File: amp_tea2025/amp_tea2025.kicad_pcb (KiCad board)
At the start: 2 copper layers, 18 parts, among them J1 in, J2 SPK, J3 SPK, U1 TEA2025

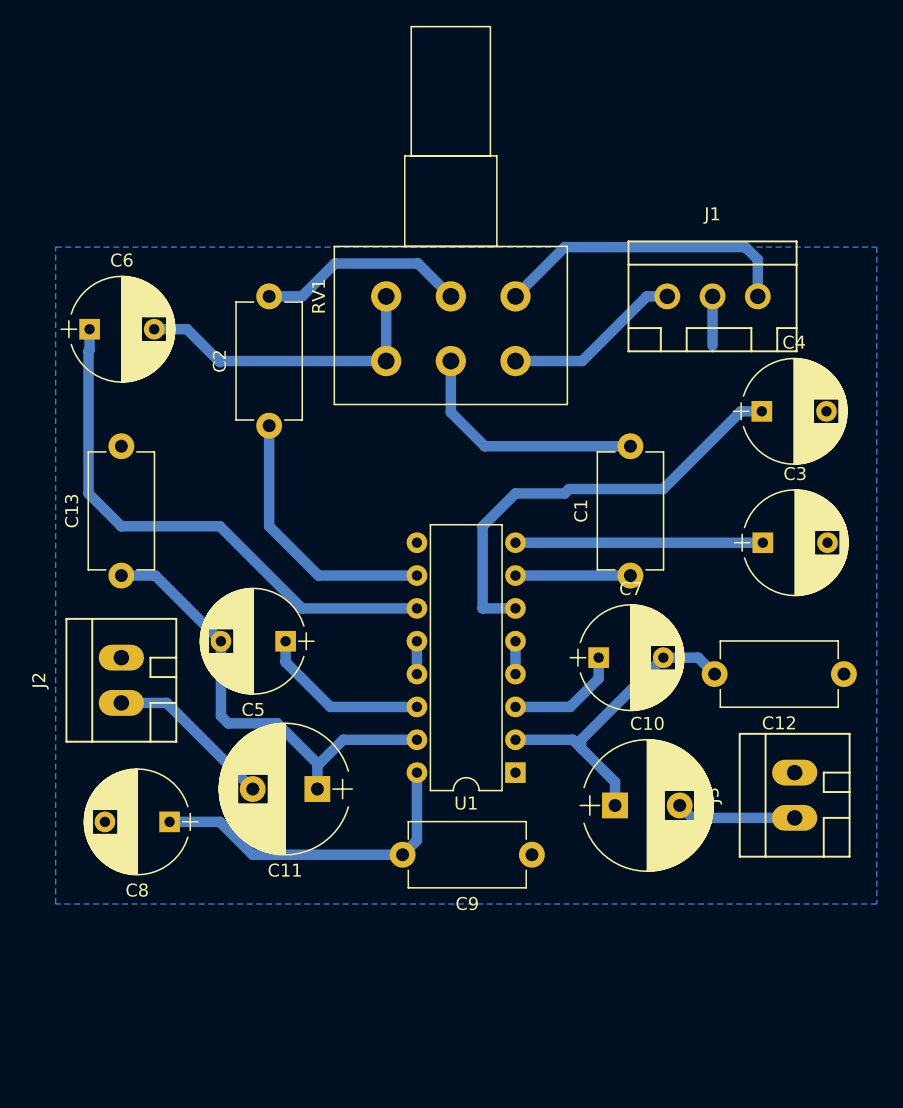
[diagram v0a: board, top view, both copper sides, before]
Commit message: pdf
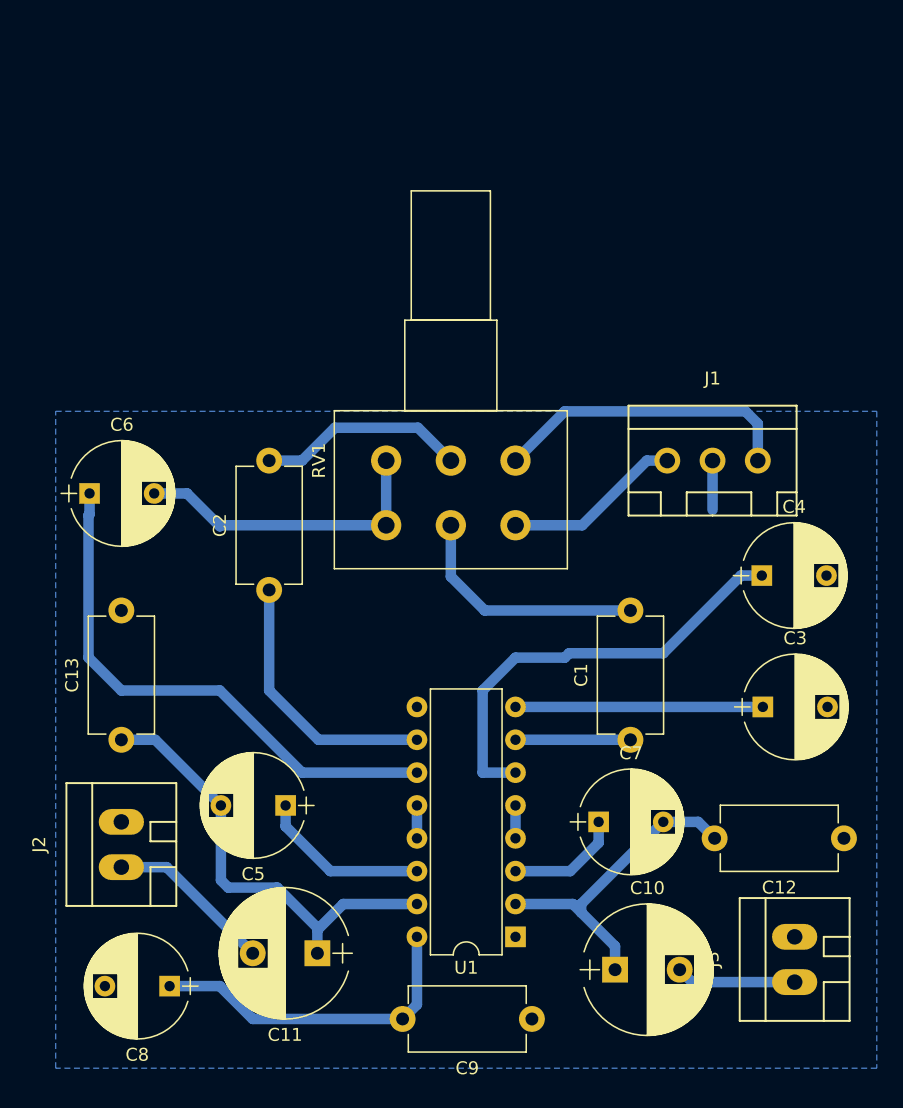
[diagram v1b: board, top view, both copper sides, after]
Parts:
- moved C11 12.7 mm to (45.6, 67.3)
- moved C12 12.7 mm to (86.4, 58.4)
- moved C4 12.7 mm to (80.0, 38.1)
- moved C5 12.7 mm to (43.2, 55.9)
- moved C9 12.7 mm to (62.2, 72.4)
- moved J2 12.7 mm to (30.5, 58.9)
- moved U1 12.7 mm to (61.0, 66.0)
- moved C2 12.7 mm to (41.9, 39.2)
- moved C6 12.7 mm to (28.0, 31.8)
- moved J1 12.7 mm to (76.2, 29.2)
- moved RV1 12.7 mm to (61.0, 29.2)
- moved C1 12.7 mm to (69.8, 50.8)
- moved C10 12.7 mm to (68.7, 68.6)
- moved C13 12.7 mm to (30.5, 50.8)
- moved C3 12.7 mm to (80.1, 48.3)
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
